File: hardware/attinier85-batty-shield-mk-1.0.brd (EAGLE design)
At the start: 36 x 25 mm, 6 parts, among them U1 ATTINIER85_SHIELDV2

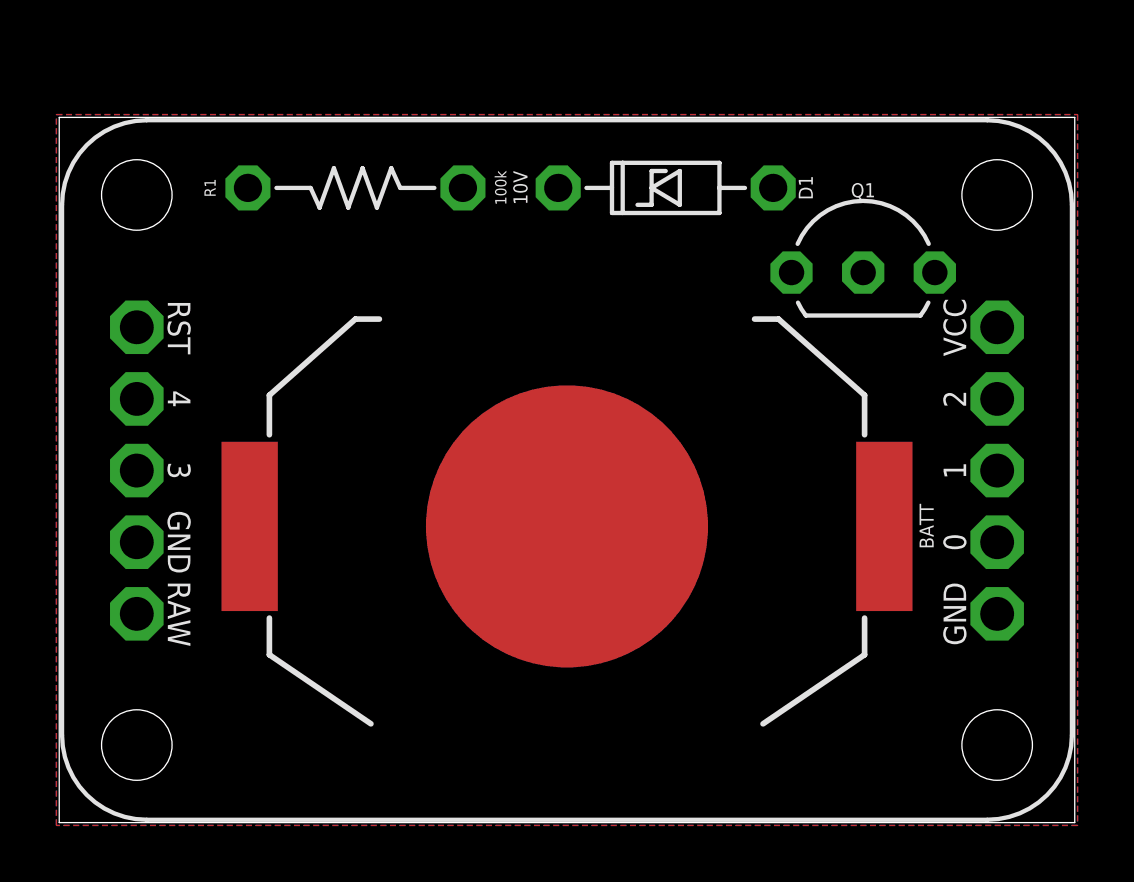
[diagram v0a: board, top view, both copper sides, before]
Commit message: cleaning up version spoo
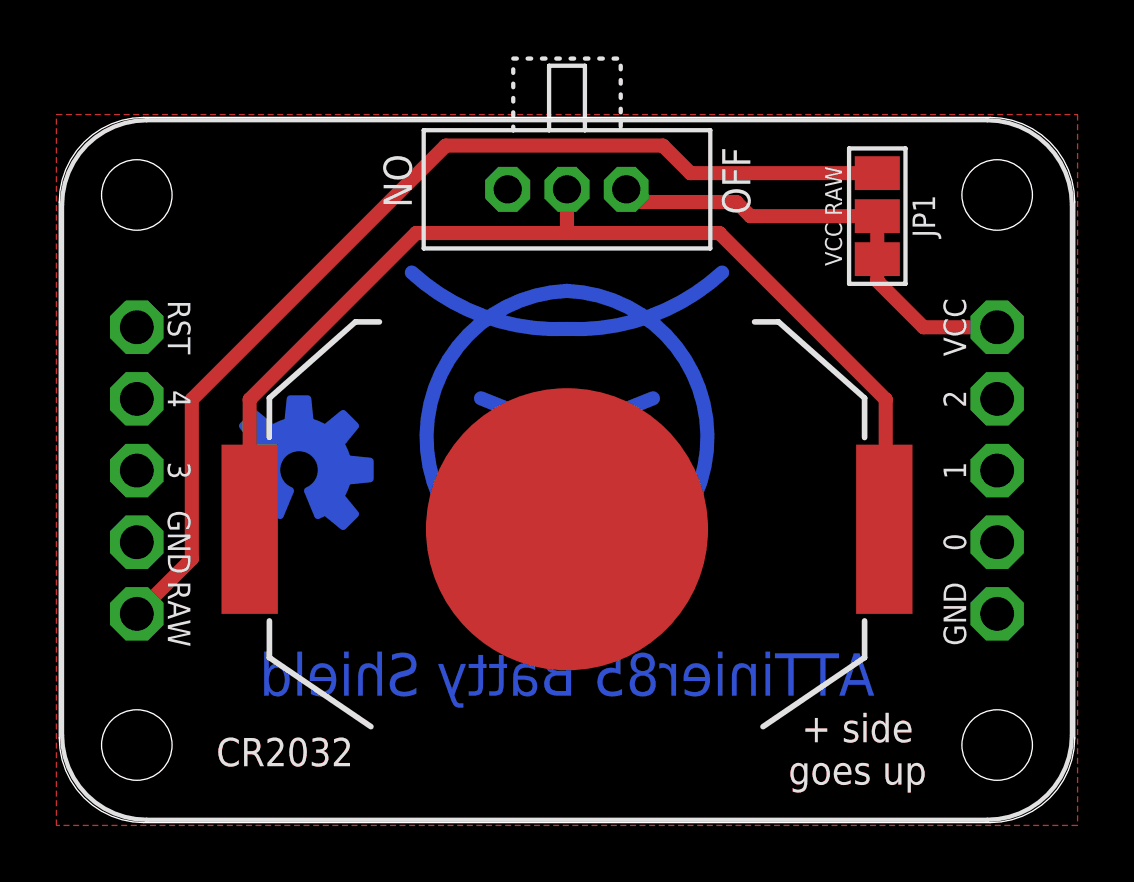
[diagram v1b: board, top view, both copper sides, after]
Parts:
- removed D1: 10V, A_butts:DIODE-ZENNER-7.62MM
- removed Q1: (no value), A_butts:TO-92-AMMO
- removed R1: 100k, A_butts:RESISTOR-AXIAL-PTH-7.62MM
- added JP1: VCC RAW, A_butts:PAD-JUMPER-3-NO_YES_SILK_FULL_BOX
- added PWR: SWITCH-SPDTPTH-RA-2MM, A_butts:SPDT-RA-2MM
- added U$3: (no value), A_butts:CC-BY-SA-4.0-NO-URL
- added U$4: (no value), A_butts:OSHWLOGO_TOP_0.2
- added U$6: (no value), A_butts:COW_METAL
- moved BATT 0.10 mm to (18.0, 10.4)
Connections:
- removed net N$1: D1.K, Q1.2, R1.P$2
- removed net V_BATT: BATT.TOP@1, D1.A, Q1.1
- new net RAW: JP1.1, U1.RAW
- new net VBATT: BATT.TOP@1, BATT.TOP@2, PWR.2
- net GND: now also U1.GND@1; no longer R1.P$1
- net VCC: now also JP1.2, JP1.3, PWR.1; no longer Q1.3
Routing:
- net VBATT: track 0.00 -> 38.2 mm
- net RAW: track 0.00 -> 36.8 mm
- net VCC: track 0.00 -> 16.5 mm
- removed copper zone on layer 16, net GND
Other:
- outline, holes or cut-outs redrawn
- board text added: "+ side goes up"
- board text added: ">AUTHOR"
- board text added: ">VERSION"
- board text added: "ATTinier85 Batty Shield"
- board text added: "CR2032"
- board text added: "OFF"
- board text added: "ON"
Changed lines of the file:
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@@
 <layer number="27" name="tValues" color="7" fill="1" visible="yes" active="yes"/>
 <layer number="28" name="bValues" color="7" fill="1" visible="yes" active="yes"/>
-<layer number="29" name="tStop" color="7" fill="3" visible="no" active="yes"/>
-<layer number="30" name="bStop" color="7" fill="6" visible="no" active="yes"/>
+<layer number="29" name="tStop" color="7" fill="3" visible="yes" active="yes"/>
+<layer number="30" name="bStop" color="7" fill="6" visible="yes" active="yes"/>
 <layer number="31" name="tCream" color="7" fill="4" visible="no" active="yes"/>
 <layer number="32" name="bCream" color="7" fill="5" visible="no" active="yes"/>
@@
 <board>
 <plain>
-<wire x1="0" y1="0" x2="36" y2="0" width="0" layer="20"/>
-<wire x1="36" y1="0" x2="36" y2="25" width="0" layer="20"/>
-<wire x1="36" y1="25" x2="0" y2="25" width="0" layer="20"/>
-<wire x1="0" y1="25" x2="0" y2="0" width="0" layer="20"/>
+<wire x1="0" y1="22" x2="0" y2="3" width="0" layer="20"/>
+<wire x1="0" y1="3" x2="3" y2="0" width="0" layer="20" curve="90"/>
+<wire x1="3" y1="0" x2="33" y2="0" width="0" layer="20"/>
+<wire x1="33" y1="0" x2="36" y2="3" width="0" layer="20" curve="90"/>
+<wire x1="36" y1="3" x2="36" y2="22" width="0" layer="20"/>
+<wire x1="36" y1="22" x2="33" y2="25" width="0" layer="20" curve="90"/>
+<wire x1="33" y1="25" x2="3" y2="25" width="0" layer="20"/>
+<wire x1="3" y1="25" x2="0" y2="22" width="0" layer="20" curve="90"/>
+<text x="12.5" y="22.75" size="1" layer="21" font="vector" ratio="16" rot="SR270" align="top-center">ON</text>
+<text x="23.5" y="22.75" size="1" layer="21" font="vector" ratio="16" rot="SR90" align="top-center">OFF</text>
+<text x="28.3" y="2.6" size="1" layer="21" font="vector" ratio="16" align="center">+ side
+goes up</text>
+<text x="18" y="6" size="1.5" layer="22" font="vector" ratio="15" rot="MR0" align="top-center">ATTinier85 Batty Shield</text>
+<text x="18" y="4" size="1" layer="22" font="vector" ratio="16" rot="MR0" align="top-center">&gt;VERSION</text>
+<text x="18" y="2.5" size="1" layer="22" font="vector" ratio="16" rot="MR0" align="top-center">&gt;AUTHOR</text>
+<text x="18" y="6" size="1.5" layer="16" font="vector" ratio="15" rot="MR0" align="top-center">ATTinier85 Batty Shield</text>
+<text x="8" y="23" size="1" layer="21" font="vector" ratio="16" align="center">&gt;VERSION</text>
+<text x="8" y="23" size="1" layer="1" font="vector" ratio="16" align="center">&gt;VERSION</text>
+<text x="28.3" y="2.6" size="1" layer="1" font="vector" ratio="16" align="center">+ side
+goes up</text>
+<text x="18" y="2.5" size="1" layer="16" font="vector" ratio="16" rot="MR0" align="top-center">&gt;AUTHOR</text>
+<text x="18" y="4" size="1" layer="16" font="vector" ratio="16" rot="MR0" align="top-center">&gt;VERSION</text>
+<text x="8" y="2.5" size="1" layer="21" font="vector" ratio="16" align="center">CR2032</text>
+<text x="8" y="2.5" size="1" layer="1" font="vector" ratio="16" align="center">CR2032</text>
 </plain>
 <attributes>
+<attribute name="AUTHOR" value="by schizobovine &lt;sean@yak.net&gt;"/>
+<attribute name="VERSION" value="Rev 1.0"/>
 </attributes>
 <variantdefs>
@@
 </element>
 <element name="U1" library="A_butts" package="ATTINIER85_SHIELD_V2" value="ATTINIER85_SHIELDV2" x="18" y="12.5"/>
-<element name="BATT" library="A_butts" package="BATTCON_20MM_MINE" value="CR2032" x="18" y="10.5" rot="R270"/>
-<element name="D1" library="A_butts" package="DIODE-ZENNER-7.62MM" value="10V" x="21.5" y="22.5" rot="R180"/>
-<element name="R1" library="A_butts" package="RESISTOR-AXIAL-PTH-7.62MM" value="100k" x="10.5" y="22.5"/>
-<element name="Q1" library="A_butts" package="TO-92-AMMO" value="" x="28.5" y="19.5"/>
+<element name="BATT" library="A_butts" package="BATTCON_20MM_MINE" value="CR2032" x="18" y="10.4" smashed="yes" rot="R270"/>
+<element name="U$3" library="A_butts" package="CC-BY-SA-4.0-NO-URL" value="" x="27.5" y="12.5" rot="MR0"/>
+<element name="U$4" library="A_butts" package="OSHWLOGO_TOP_0.2" value="" x="8.5" y="12.5" rot="MR0"/>
+<element name="U$6" library="A_butts" package="COW_METAL" value="" x="18" y="12.5" rot="MR0"/>
+<element name="PWR" library="A_butts" package="SPDT-RA-2MM" value="SWITCH-SPDTPTH-RA-2MM" x="18" y="22.45" smashed="yes" rot="R180"/>
+<element name="JP1" library="A_butts" package="PAD-JUMPER-3-NO_YES_SILK_FULL_BOX" value="VCC   RAW" x="29" y="21.5" smashed="yes" rot="R270">
+<attribute name="NAME" x="30.25" y="21.5" size="0.8" layer="25" font="vector" ratio="12" rot="R270" align="bottom-center"/>
+<attribute name="VALUE" x="27.75" y="21.5" size="0.6" layer="21" font="vector" ratio="12" rot="R270" align="top-center"/>
+</element>
 </elements>
 <signals>
@@
 <vertex x="36.1" y="-0.1"/>
 </polygon>
-<polygon width="0.1524" layer="16">
-<vertex x="-0.1" y="-0.1"/>
-<vertex x="-0.1" y="25.1"/>
-<vertex x="36.1" y="25.1"/>
-<vertex x="36.1" y="-0.1"/>
-</polygon>
 <contactref element="BATT" pad="BOTTOM"/>
-<contactref element="R1" pad="P$1"/>
 <contactref element="U1" pad="GND@2"/>
+<contactref element="U1" pad="GND@1"/>
 </signal>
-<signal name="V_BATT">
-<contactref element="Q1" pad="1"/>
-<contactref element="D1" pad="A"/>
+<signal name="VBATT">
+<contactref element="BATT" pad="TOP@2"/>
 <contactref element="BATT" pad="TOP@1"/>
-<wire x1="25.31" y1="22.5" x2="25.96" y2="19.5" width="0" layer="19" extent="1-1"/>
-<wire x1="29.25" y1="10.5" x2="25.96" y2="19.5" width="0" layer="19" extent="1-1"/>
+<contactref element="PWR" pad="2"/>
+<wire x1="6.75" y1="10.4" x2="6.75" y2="15" width="0.5" layer="1"/>
+<wire x1="6.75" y1="15" x2="12.65" y2="20.9" width="0.5" layer="1"/>
+<wire x1="12.65" y1="20.9" x2="18" y2="20.9" width="0.5" layer="1"/>
+<wire x1="18" y1="20.9" x2="18" y2="22.45" width="0.5" layer="1"/>
+<wire x1="29.25" y1="10.4" x2="29.3" y2="10.45" width="0.5" layer="1"/>
+<wire x1="29.3" y1="10.45" x2="29.3" y2="15" width="0.5" layer="1"/>
+<wire x1="18" y1="20.9" x2="23.4" y2="20.9" width="0.5" layer="1"/>
+<wire x1="23.4" y1="20.9" x2="29.3" y2="15" width="0.5" layer="1"/>
+</signal>
+<signal name="RAW">
+<contactref element="U1" pad="RAW"/>
+<contactref element="JP1" pad="1"/>
+<wire x1="29" y1="23.024" x2="22.376" y2="23.024" width="0.5" layer="1"/>
+<wire x1="22.376" y1="23.024" x2="21.4" y2="24" width="0.5" layer="1"/>
+<wire x1="2.75" y1="7.4" x2="4.7" y2="9.35" width="0.5" layer="1"/>
+<wire x1="4.7" y1="9.35" x2="4.7" y2="15" width="0.5" layer="1"/>
+<wire x1="4.7" y1="15" x2="13.7" y2="24" width="0.5" layer="1"/>
+<wire x1="13.7" y1="24" x2="21.4" y2="24" width="0.5" layer="1"/>
 </signal>
 <signal name="VCC">
 <contactref element="U1" pad="VCC"/>
-<contactref element="Q1" pad="3"/>
-<wire x1="31.04" y1="19.5" x2="33.25" y2="17.56" width="0" layer="19" extent="1-1"/>
-</signal>
-<signal name="N$1">
-<contactref element="R1" pad="P$2"/>
-<contactref element="Q1" pad="2"/>
-<contactref element="D1" pad="K"/>
-<wire x1="17.69" y1="22.5" x2="28.5" y2="19.5" width="0" layer="19" extent="1-1"/>
-<wire x1="14.31" y1="22.5" x2="17.69" y2="22.5" width="0" layer="19" extent="1-1"/>
+<contactref element="JP1" pad="3"/>
+<contactref element="PWR" pad="1"/>
+<contactref element="JP1" pad="2"/>
+<wire x1="20.1" y1="22.45" x2="20.55" y2="22" width="0.5" layer="1"/>
+<wire x1="20.55" y1="22" x2="24" y2="22" width="0.5" layer="1"/>
+<wire x1="24" y1="22" x2="24.5" y2="21.5" width="0.5" layer="1"/>
+<wire x1="24.5" y1="21.5" x2="29" y2="21.5" width="0.5" layer="1"/>
+<wire x1="29" y1="21.5" x2="29" y2="19.976" width="0.5" layer="1"/>
+<wire x1="30.64" y1="17.56" x2="33.25" y2="17.56" width="0.5" layer="1"/>
+<wire x1="29" y1="19.976" x2="29" y2="19.2" width="0.5" layer="1"/>
+<wire x1="29" y1="19.2" x2="30.64" y2="17.56" width="0.5" layer="1"/>
 </signal>
 </signals>
 </board>
 </drawing>
+<compatibility>
+<note version="6.3" minversion="6.2.2" severity="warning">
+Since Version 6.2.2 text objects can contain more than one line,
+which will not be processed correctly with this version.
+</note>
+</compatibility>
 </eagle>
